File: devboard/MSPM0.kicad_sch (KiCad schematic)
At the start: 66 parts, among them J1 USB_C_USB2.0, J2 SWD, J3 Conn_01x03_Pin, J4 Conn_01x02, J5 Conn_01x03_Pin, J6 Conn_01x08_Power, J7 Conn_01x06_Analog, J8 Conn_01x08_DigitalLow, J9 Conn_01x10_DigitalHigh, SW1 SW, SW2 SW_Push, SW3 SW, SW4 SW_Push, SW5 SW_Push, U2 AP2112K-3.3, Y2 40MHz

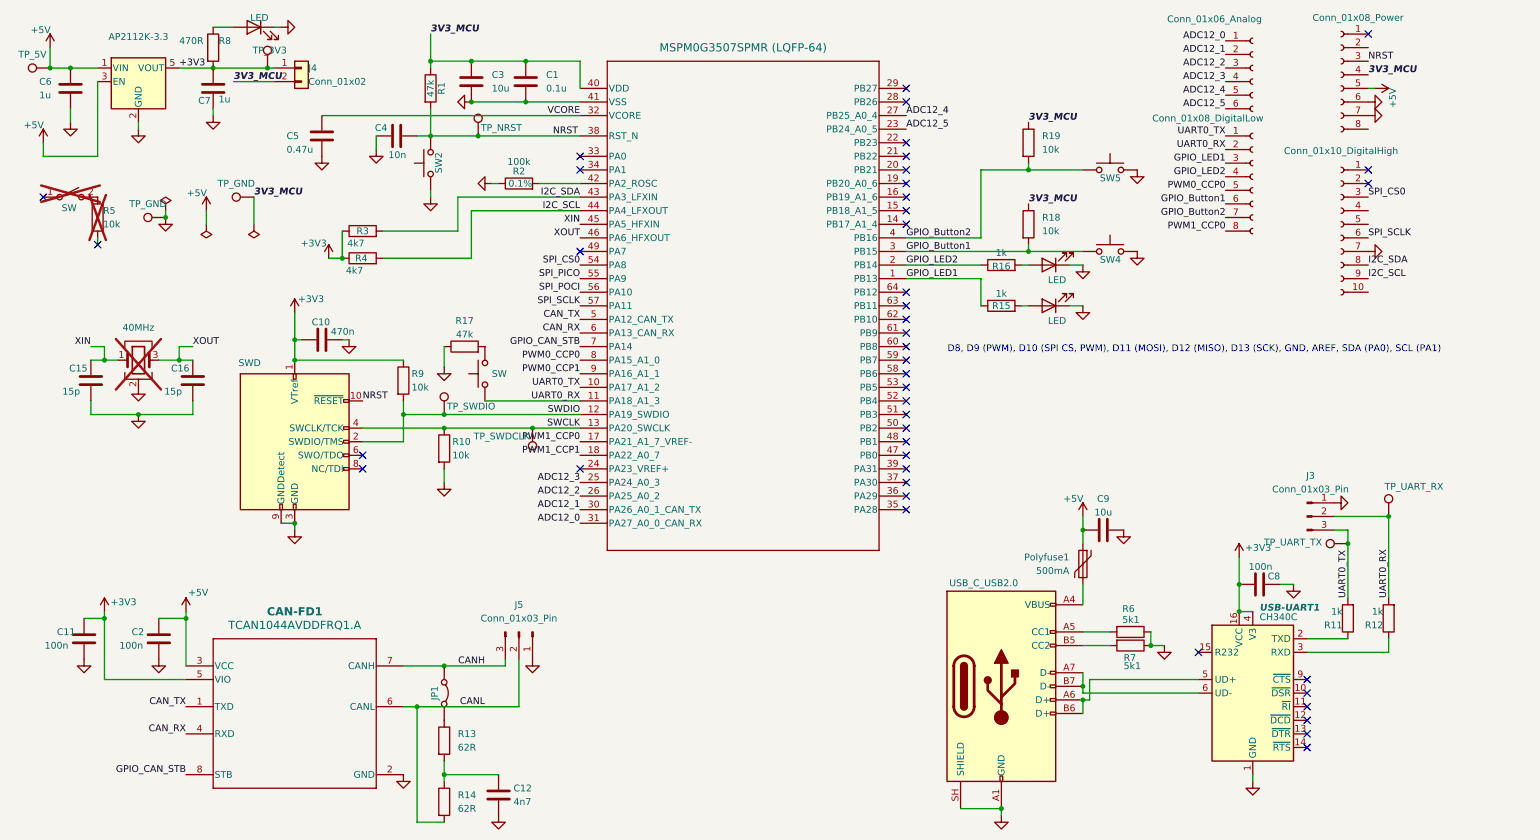
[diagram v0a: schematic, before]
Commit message: headers done, let's proofcheck all the schematic
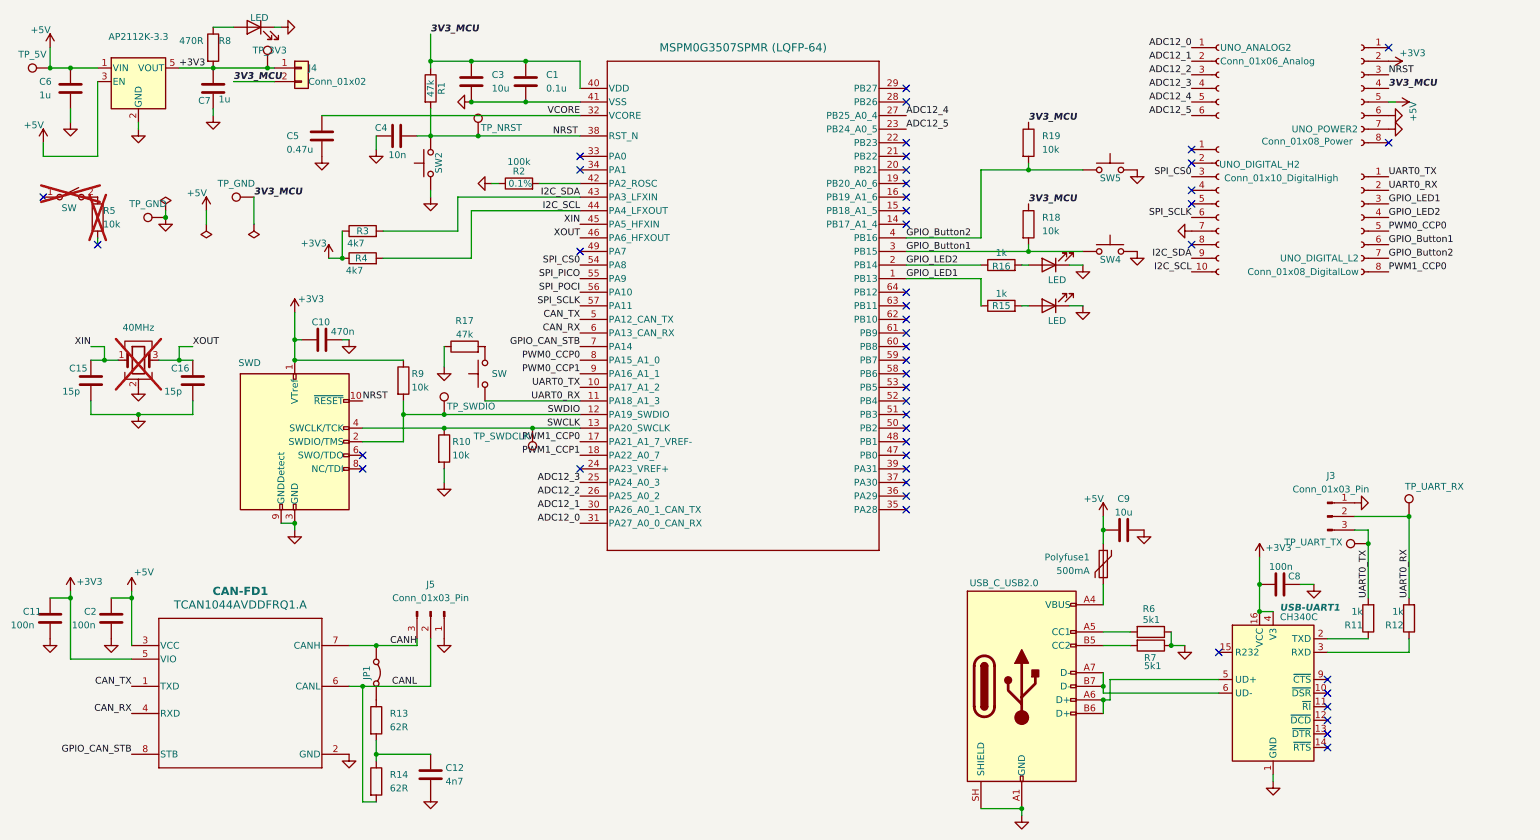
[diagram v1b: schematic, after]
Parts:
- removed J6: Conn_01x08_Power, symbol Connector:Conn_01x08_Socket
- removed J7: Conn_01x06_Analog, symbol Connector:Conn_01x06_Socket
- removed J8: Conn_01x08_DigitalLow, symbol Connector:Conn_01x08_Socket
- removed J9: Conn_01x10_DigitalHigh, symbol Connector:Conn_01x10_Socket
- added UNO_ANALOG2: Conn_01x06_Analog, Connector_PinSocket_2.54mm:PinSocket_1x06_P2.54mm_Vertical, symbol Connector:Conn_01x06_Socket
- added UNO_DIGITAL_H2: Conn_01x10_DigitalHigh, Connector_PinSocket_2.54mm:PinSocket_1x10_P2.54mm_Vertical, symbol Connector:Conn_01x10_Socket
- added UNO_DIGITAL_L2: Conn_01x08_DigitalLow, Connector_PinSocket_2.54mm:PinSocket_1x08_P2.54mm_Vertical, symbol Connector:Conn_01x08_Socket
- added UNO_POWER2: Conn_01x08_Power, Connector_PinSocket_2.54mm:PinSocket_1x08_P2.54mm_Vertical, symbol Connector:Conn_01x08_Socket
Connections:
- net +3V3: now also UNO_POWER2.2 (Pin_2)
- net +5V: now also UNO_POWER2.5 (Pin_5)
- net 3V3_MCU: now also UNO_POWER2.4 (Pin_4)
- net ADC12_0: now also UNO_ANALOG2.1 (Pin_1)
- net ADC12_1: now also UNO_ANALOG2.2 (Pin_2)
- net ADC12_2: now also UNO_ANALOG2.3 (Pin_3)
- net ADC12_3: now also UNO_ANALOG2.4 (Pin_4)
- net ADC12_4: now also UNO_ANALOG2.5 (Pin_5)
- net ADC12_5: now also UNO_ANALOG2.6 (Pin_6)
- net GND: now also UNO_DIGITAL_H2.7 (Pin_7), UNO_POWER2.6 (Pin_6), UNO_POWER2.7 (Pin_7)
- net GPIO_Button1: now also UNO_DIGITAL_L2.6 (Pin_6)
- net GPIO_Button2: now also UNO_DIGITAL_L2.7 (Pin_7)
- net GPIO_LED1: now also UNO_DIGITAL_L2.3 (Pin_3)
- net GPIO_LED2: now also UNO_DIGITAL_L2.4 (Pin_4)
- net I2C_SCL: now also UNO_DIGITAL_H2.10 (Pin_10)
- net I2C_SDA: now also UNO_DIGITAL_H2.9 (Pin_9)
- net NRST: now also UNO_POWER2.3 (Pin_3)
- net PWM0_CCP0: now also UNO_DIGITAL_L2.5 (Pin_5)
- net PWM1_CCP0: now also UNO_DIGITAL_L2.8 (Pin_8)
- net SPI_CS0: now also UNO_DIGITAL_H2.3 (Pin_3)
- net SPI_SCLK: now also UNO_DIGITAL_H2.6 (Pin_6)
- net UART0_RX: now also UNO_DIGITAL_L2.2 (Pin_2)
- net UART0_TX: now also UNO_DIGITAL_L2.1 (Pin_1)
- no-connect marks 44 -> 48
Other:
- note removed: "D8, D9 (PWM), D10 (SPI CS, PWM), D11 (MOSI), D12 (MISO), D13 (SCK), GND, AREF, SDA (PA0), SCL (PA1)"
- moved on the sheet: C11, C12, C2, C8, C9, CAN-FD1, J3, J5, JP1, Polyfuse1, R11, R12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
